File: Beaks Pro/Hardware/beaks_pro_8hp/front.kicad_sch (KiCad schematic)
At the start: 30 parts, among them J11 out1, J12 out2, J2 Pins_02x10_P2.54mm_TH, J3 CV1, J4 CV2, J5 CV3, J6 CV4, J7 in1, J8 in2, J9 Pins_02x10_P2.54mm_TH, SW2 SW_Dual, SW3 SW_Mode, SW5 SW_ML6, SW6 SW_ML6

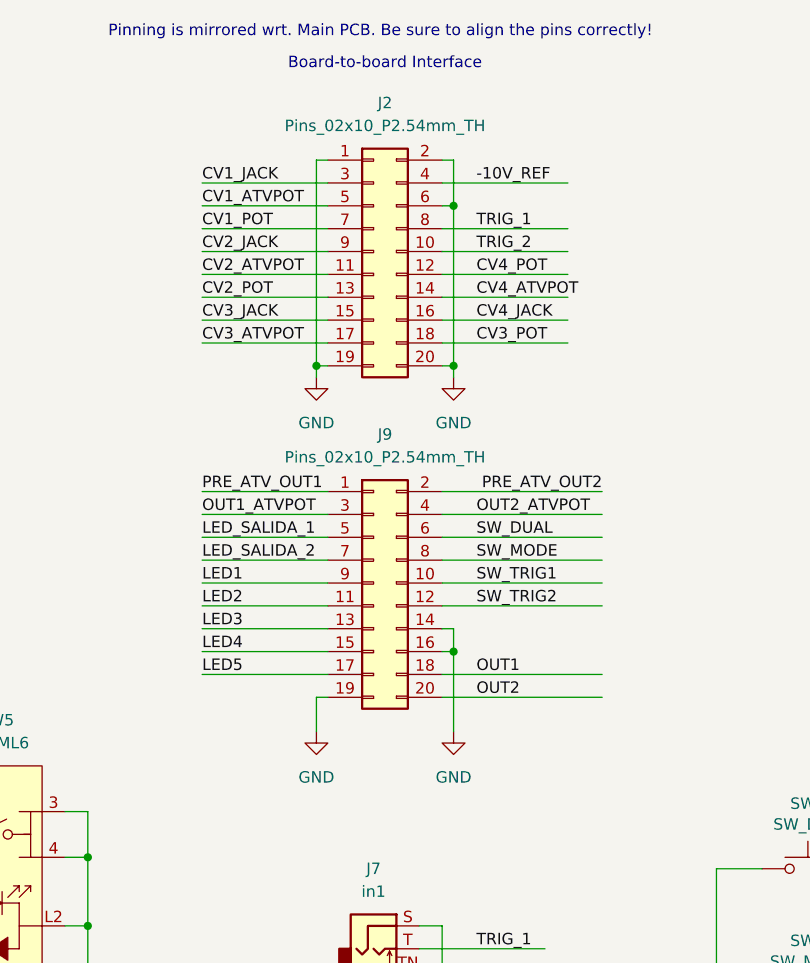
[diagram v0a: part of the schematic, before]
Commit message: Layout done on 8HP SMT version
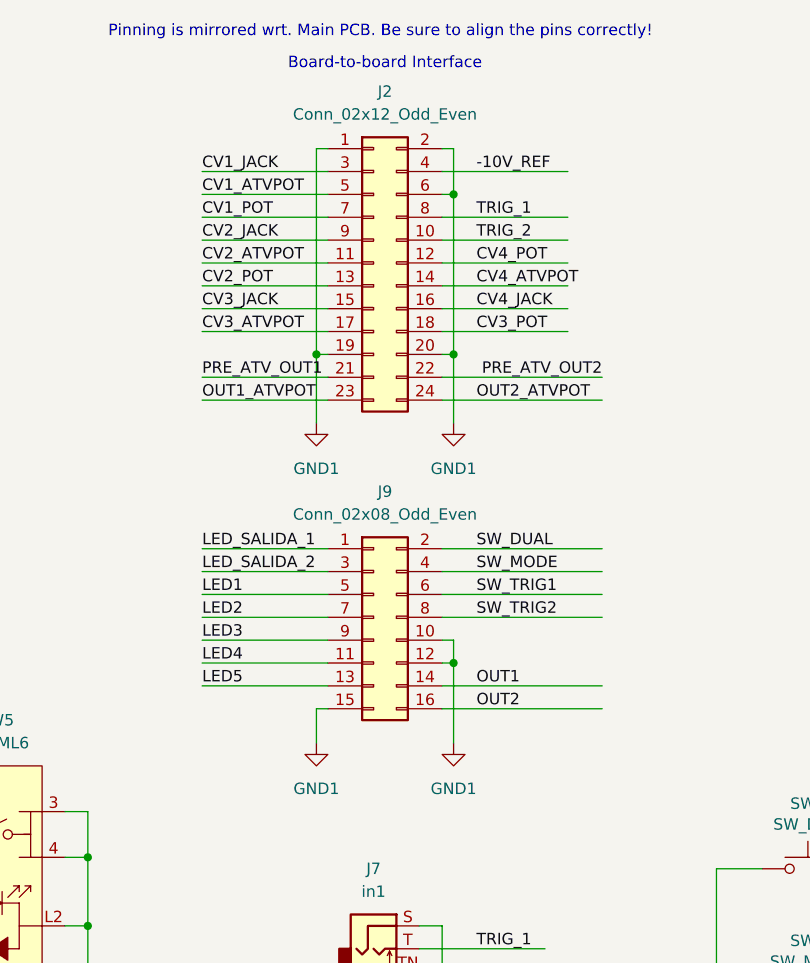
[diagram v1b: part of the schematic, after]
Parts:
- removed J2, J9: Pins_02x10_P2.54mm_TH, Connector_PinSocket_2.54mm:PinSocket_2x10_P2.54mm_Vertical, symbol PCM_4ms_Connector:Pins_02x10_P1.27mm_TH
- added J2: Conn_02x12_Odd_Even, Connector_PinHeader_2.54mm:PinHeader_2x12_P2.54mm_Vertical, symbol Connector_Generic:Conn_02x12_Odd_Even
- added J9: Conn_02x08_Odd_Even, Connector_PinHeader_2.54mm:PinHeader_2x08_P2.54mm_Vertical, symbol Connector_Generic:Conn_02x08_Odd_Even
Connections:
- net -10V_REF: now also J2.4 (Pin_4)
- net CV1_ATVPOT: now also J2.5 (Pin_5)
- net CV1_JACK: now also J2.3 (Pin_3)
- net CV1_POT: now also J2.7 (Pin_7)
- net CV2_ATVPOT: now also J2.11 (Pin_11)
- net CV2_JACK: now also J2.9 (Pin_9)
- net CV2_POT: now also J2.13 (Pin_13)
- net CV3_ATVPOT: now also J2.17 (Pin_17)
- net CV3_JACK: now also J2.15 (Pin_15)
- net CV3_POT: now also J2.18 (Pin_18)
- net CV4_ATVPOT: now also J2.14 (Pin_14)
- net CV4_JACK: now also J2.16 (Pin_16)
- net CV4_POT: now also J2.12 (Pin_12)
- net GND1: now also J2.1 (Pin_1), J2.19 (Pin_19), J2.2 (Pin_2), J2.20 (Pin_20), J2.6 (Pin_6), J9.10 (Pin_10), J9.12 (Pin_12), J9.15 (Pin_15)
- net LED1: now also J9.5 (Pin_5)
- net LED2: now also J9.7 (Pin_7)
- net LED3: now also J9.9 (Pin_9)
- net LED4: now also J9.11 (Pin_11)
- net LED5: now also J9.13 (Pin_13)
- net LED_SALIDA_1: now also J9.1 (Pin_1)
- net LED_SALIDA_2: now also J9.3 (Pin_3)
- net OUT1: now also J9.14 (Pin_14)
- net OUT1_ATVPOT: now also J2.23 (Pin_23)
- net OUT2: now also J9.16 (Pin_16)
- net OUT2_ATVPOT: now also J2.24 (Pin_24)
- net PRE_ATV_OUT1: now also J2.21 (Pin_21)
- net PRE_ATV_OUT2: now also J2.22 (Pin_22)
- net SW_DUAL: now also J9.2 (Pin_2)
- net SW_MODE: now also J9.4 (Pin_4)
- net SW_TRIG1: now also J9.6 (Pin_6)
- net SW_TRIG2: now also J9.8 (Pin_8)
- net TRIG_1: now also J2.8 (Pin_8)
- net TRIG_2: now also J2.10 (Pin_10)
